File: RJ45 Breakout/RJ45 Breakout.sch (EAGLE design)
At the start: 6 parts, among them J1 RJ45-8X, X1 

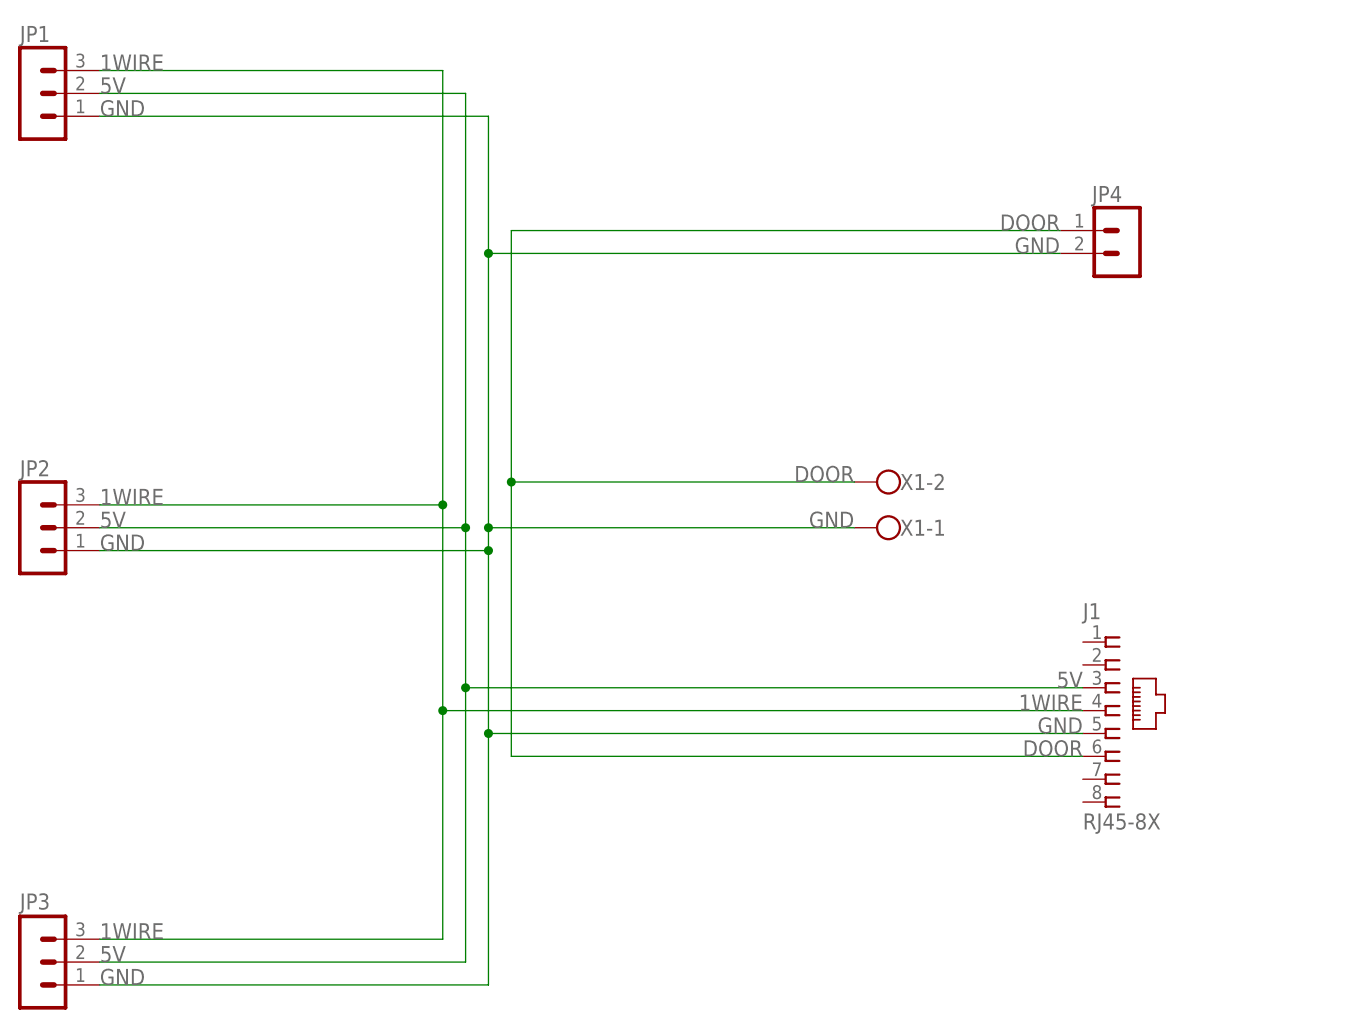
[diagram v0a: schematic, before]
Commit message: Add RJ45 Breakout
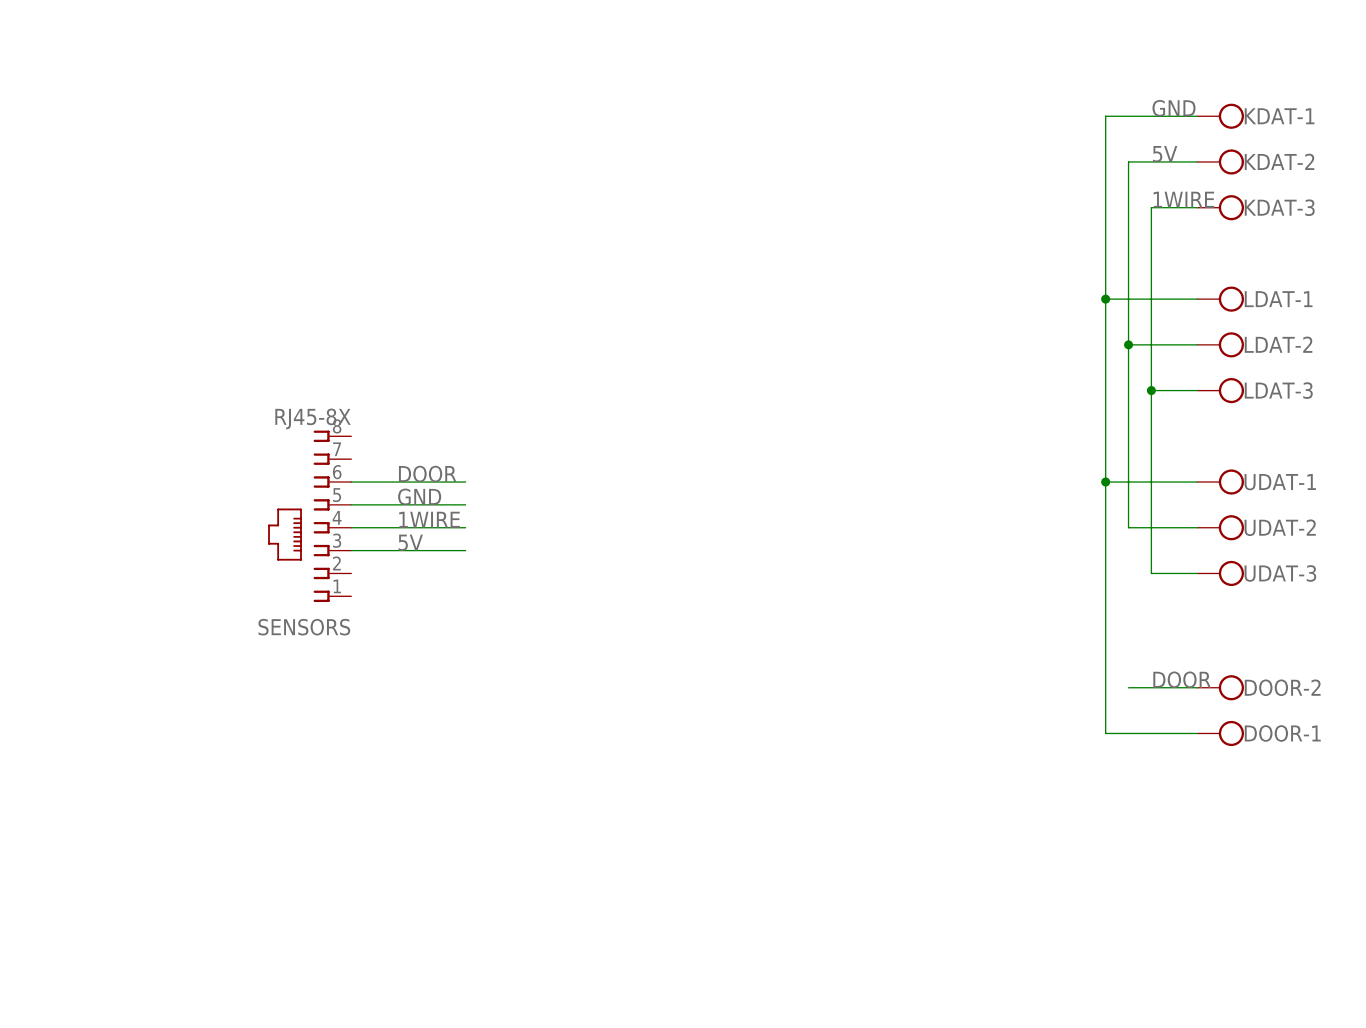
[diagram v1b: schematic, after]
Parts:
- removed J1: RJ45-8X, con-tycoelectronics:RJ45-8X
- removed JP1, JP2: (no value), Donnie:HDR-3
- removed JP3: OneWire, Donnie:HDR-3
- removed JP4: HDR-2, Donnie:HDR-2
- removed X1: (no value), con-wago-500:W237-102
- added DOOR: (no value), con-wago-500:W237-102
- added KDAT, LDAT, UDAT: (no value), con-wago-500:W237-103
- added SENSORS: RJ45-8X, con-tycoelectronics:RJ45-8X
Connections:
- net 1WIRE: now also KDAT-3.KL, LDAT-3.KL, SENSORS.4, UDAT-3.KL; no longer J1.4, JP1.3, JP2.3, JP3.3
- net 5V: now also KDAT-2.KL, LDAT-2.KL, SENSORS.3, UDAT-2.KL; no longer J1.3, JP1.2, JP2.2, JP3.2
- net DOOR: now also DOOR-2.KL, SENSORS.6; no longer J1.6, JP4.1, X1-2.KL
- net GND: now also DOOR-1.KL, KDAT-1.KL, LDAT-1.KL, SENSORS.5, UDAT-1.KL; no longer J1.5, JP1.1, JP2.1, JP3.1, JP4.2, X1-1.KL
